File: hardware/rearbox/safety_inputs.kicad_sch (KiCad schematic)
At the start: 9 parts, among them U9 TCA6416ARTWR

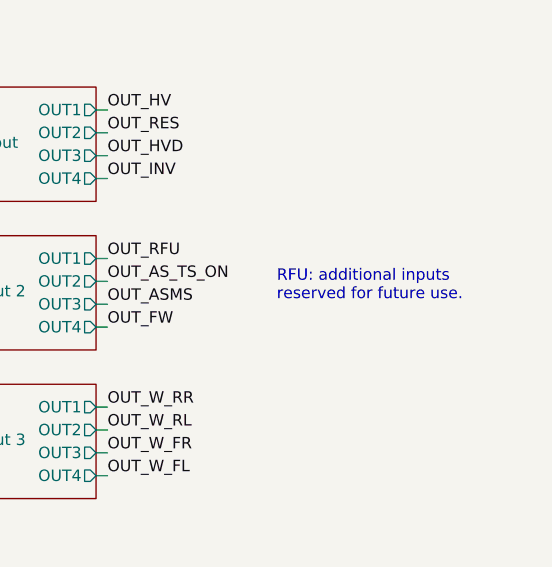
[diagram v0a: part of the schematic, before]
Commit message: Changed power section
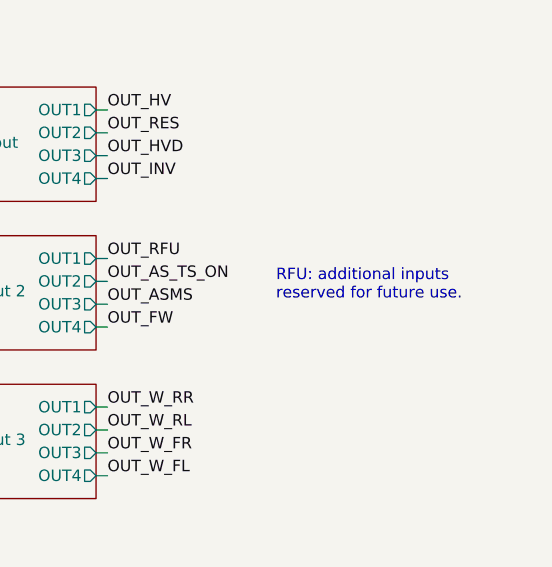
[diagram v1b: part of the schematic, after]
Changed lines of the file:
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@@
 (kicad_sch
-	(version 20231120)
+	(version 20250114)
 	(generator "eeschema")
-	(generator_version "8.0")
+	(generator_version "9.0")
 	(paper "A4")
 	(title_block
@@
 		(comment 1 "Reviewer:")
 	)
+	(text "Status\n LEDs\n"
+		(exclude_from_sim no)
+		(at 174.244 108.204 90)
+		(effects
+			(font
+				(size 1.27 1.27)
+			)
+			(justify left bottom)
+		)
+	)
+	(text_box "RFU: additional inputs reserved for future use."
+		(exclude_from_sim no)
+		(at 248.92 93.98 0)
+		(size 29.21 5.08)
+		(margins 0.9524 0.9524 0.9524 0.9524)
+		(stroke
+			(width -0.0001)
+			(type default)
+		)
+		(fill
+			(type none)
+		)
+		(effects
+			(font
+				(size 1.27 1.27)
+			)
+			(justify left top)
+		)
+	)
 	(junction
 		(at 66.04 104.14)
@@
 		)
 	)
-	(text_box "RFU: additional inputs reserved for future use."
-		(exclude_from_sim no)
-		(at 248.92 93.98 0)
-		(size 29.21 5.08)
-		(stroke
-			(width -0.0001)
-			(type default)
-		)
-		(fill
-			(type none)
-		)
-		(effects
-			(font
-				(size 1.27 1.27)
-			)
-			(justify left top)
-		)
-	)
-	(text "Status\n LEDs\n"
-		(exclude_from_sim no)
-		(at 174.244 108.204 90)
-		(effects
-			(font
-				(size 1.27 1.27)
-			)
-			(justify left bottom)
-		)
-	)
 	(label "OUT_INV"
 		(at 231.14 85.09 0)
-		(fields_autoplaced yes)
 		(effects
 			(font
@@
 	(label "OUT_W_RR"
 		(at 231.14 110.49 0)
-		(fields_autoplaced yes)
 		(effects
 			(font
@@
 	(label "OUT_RES"
 		(at 231.14 80.01 0)
-		(fields_autoplaced yes)
 		(effects
 			(font
@@
 	(label "OUT_W_FL"
 		(at 154.94 111.76 0)
-		(fields_autoplaced yes)
 		(effects
 			(font
@@
 	(label "OUT_ASMS"
 		(at 154.94 83.82 0)
-		(fields_autoplaced yes)
 		(effects
 			(font
@@
 	(label "OUT_HVD"
 		(at 231.14 82.55 0)
-		(fields_autoplaced yes)
 		(effects
 			(font
@@
 	(label "OUT_W_FR"
 		(at 231.14 115.57 0)
-		(fields_autoplaced yes)
 		(effects
 			(font
@@
 	(label "OUT_ASMS"
 		(at 231.14 99.06 0)
-		(fields_autoplaced yes)
 		(effects
 			(font
@@
 	(label "OUT_FW"
 		(at 231.14 101.6 0)
-		(fields_autoplaced yes)
 		(effects
 			(font
@@
 	(label "OUT_FW"
 		(at 154.94 86.36 0)
-		(fields_autoplaced yes)
 		(effects
 			(font
@@
 	(label "TCA_VDD"
 		(at 138.43 69.85 90)
-		(fields_autoplaced yes)
 		(effects
 			(font
@@
 	(label "OUT_HV"
 		(at 231.14 77.47 0)
-		(fields_autoplaced yes)
 		(effects
 			(font
@@
 	(label "OUT_HV"
 		(at 154.94 88.9 0)
-		(fields_autoplaced yes)
 		(effects
 			(font
@@
 	(label "OUT_AS_TS_ON"
 		(at 231.14 96.52 0)
-		(fields_autoplaced yes)
 		(effects
 			(font
@@
 	(label "OUT_AS_TS_ON"
 		(at 154.94 81.28 0)
-		(fields_autoplaced yes)
 		(effects
 			(font
@@
 	(label "OUT_W_RL"
 		(at 231.14 113.03 0)
-		(fields_autoplaced yes)
 		(effects
 			(font
@@
 	(label "OUT_RFU"
 		(at 154.94 78.74 0)
-		(fields_autoplaced yes)
 		(effects
 			(font
@@
 	(label "OUT_W_FL"
 		(at 231.14 118.11 0)
-		(fields_autoplaced yes)
 		(effects
 			(font
@@
 	(label "TCA_VDD"
 		(at 73.66 96.52 0)
-		(fields_autoplaced yes)
 		(effects
 			(font
@@
 	(label "OUT_W_RL"
 		(at 154.94 116.84 0)
-		(fields_autoplaced yes)
 		(effects
 			(font
@@
 	(label "OUT_RES"
 		(at 154.94 91.44 0)
-		(fields_autoplaced yes)
 		(effects
 			(font
@@
 	(label "OUT_HVD"
 		(at 154.94 93.98 0)
-		(fields_autoplaced yes)
 		(effects
 			(font
@@
 	(label "OUT_INV"
 		(at 154.94 96.52 0)
-		(fields_autoplaced yes)
 		(effects
 			(font
@@
 	(label "OUT_W_RR"
 		(at 154.94 119.38 0)
-		(fields_autoplaced yes)
 		(effects
 			(font
@@
 	(label "OUT_RFU"
 		(at 231.14 93.98 0)
-		(fields_autoplaced yes)
 		(effects
 			(font
@@
 	(label "OUT_W_FR"
 		(at 154.94 114.3 0)
-		(fields_autoplaced yes)
 		(effects
 			(font
@@
 		(shape input)
 		(at 201.93 85.09 180)
-		(fields_autoplaced yes)
 		(effects
 			(font
@@
 		(shape input)
 		(at 201.93 93.98 180)
-		(fields_autoplaced yes)
 		(effects
 			(font
@@
 		(shape input)
 		(at 201.93 115.57 180)
-		(fields_autoplaced yes)
 		(effects
 			(font
@@
 		(shape bidirectional)
 		(at 105.41 85.09 180)
-		(fields_autoplaced yes)
 		(effects
 			(font
@@
 		(shape input)
 		(at 105.41 82.55 180)
-		(fields_autoplaced yes)
 		(effects
 			(font
@@
 		(shape input)
 		(at 201.93 118.11 180)
-		(fields_autoplaced yes)
 		(effects
 			(font
@@
 		(shape output)
 		(at 154.94 104.14 0)
-		(fields_autoplaced yes)
 		(effects
 			(font
@@
 		(shape input)
 		(at 201.93 101.6 180)
-		(fields_autoplaced yes)
 		(effects
 			(font
@@
 		(shape input)
 		(at 201.93 110.49 180)
-		(fields_autoplaced yes)
 		(effects
 			(font
@@
 		(shape input)
 		(at 201.93 77.47 180)
-		(fields_autoplaced yes)
 		(effects
 			(font
@@
 		(shape input)
 		(at 201.93 96.52 180)
-		(fields_autoplaced yes)
 		(effects
 			(font
@@
 		(shape input)
 		(at 201.93 82.55 180)
-		(fields_autoplaced yes)
 		(effects
 			(font
@@
 		(shape output)
 		(at 154.94 101.6 0)
-		(fields_autoplaced yes)
 		(effects
 			(font
@@
 		(shape input)
 		(at 201.93 99.06 180)
-		(fields_autoplaced yes)
 		(effects
 			(font
@@
 		(shape input)
 		(at 201.93 113.03 180)
-		(fields_autoplaced yes)
 		(effects
 			(font
@@
 		(shape output)
 		(at 154.94 106.68 0)
-		(fields_autoplaced yes)
 		(effects
 			(font
@@
 		(shape output)
 		(at 105.41 90.17 180)
-		(fields_autoplaced yes)
 		(effects
 			(font
@@
 		(shape input)
 		(at 105.41 87.63 180)
-		(fields_autoplaced yes)
 		(effects
 			(font
@@
 		(shape input)
 		(at 201.93 80.01 180)
-		(fields_autoplaced yes)
 		(effects
 			(font
@@
 		(at 203.2 107.95)
 		(size 26.67 12.7)
+		(exclude_from_sim no)
+		(in_bom yes)
+		(on_board yes)
+		(dnp no)
 		(stroke
 			(width 0.1524)
@@
 		(at 203.2 74.93)
 		(size 26.67 12.7)
+		(exclude_from_sim no)
+		(in_bom yes)
+		(on_board yes)
+		(dnp no)
 		(stroke
 			(width 0.1524)
@@
 		(at 203.2 91.44)
 		(size 26.67 12.7)
+		(exclude_from_sim no)
+		(in_bom yes)
+		(on_board yes)
+		(dnp no)
 		(stroke
 			(width 0.1524)
